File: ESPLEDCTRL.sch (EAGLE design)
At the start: 15 parts, among them IC1 74HC1G08GW

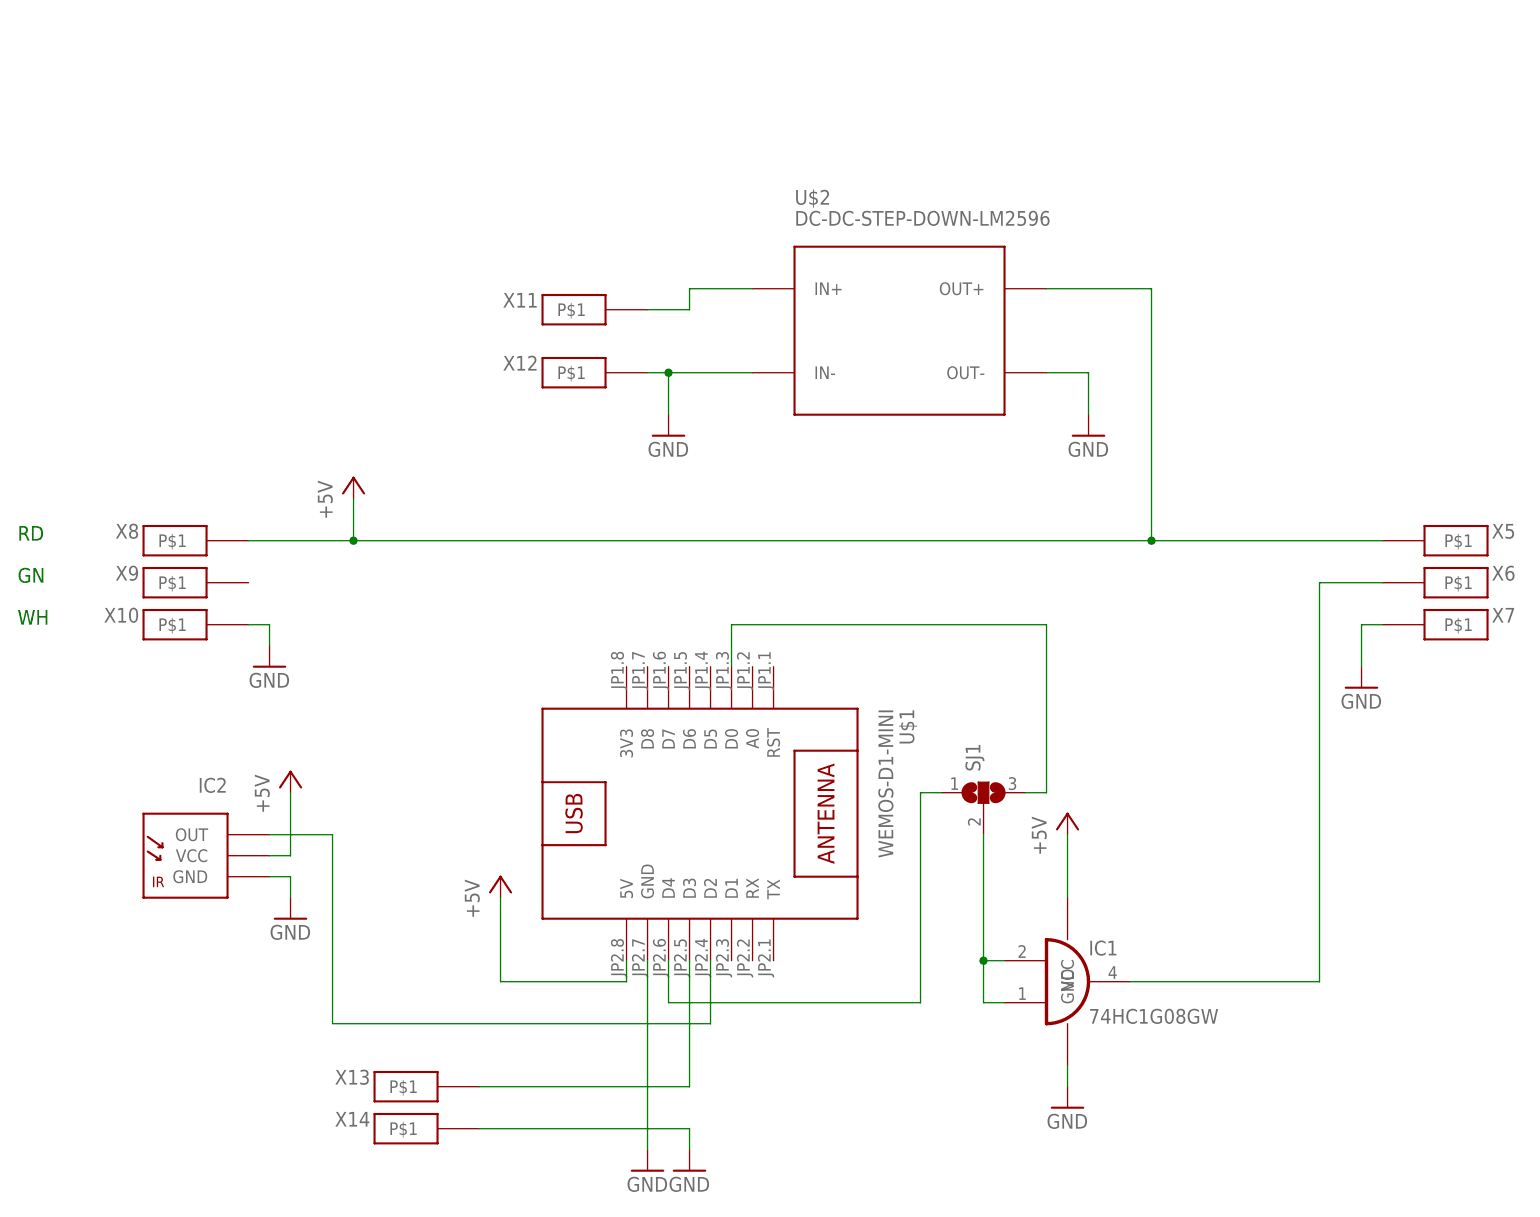
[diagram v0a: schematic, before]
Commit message: Board fertig gestellt
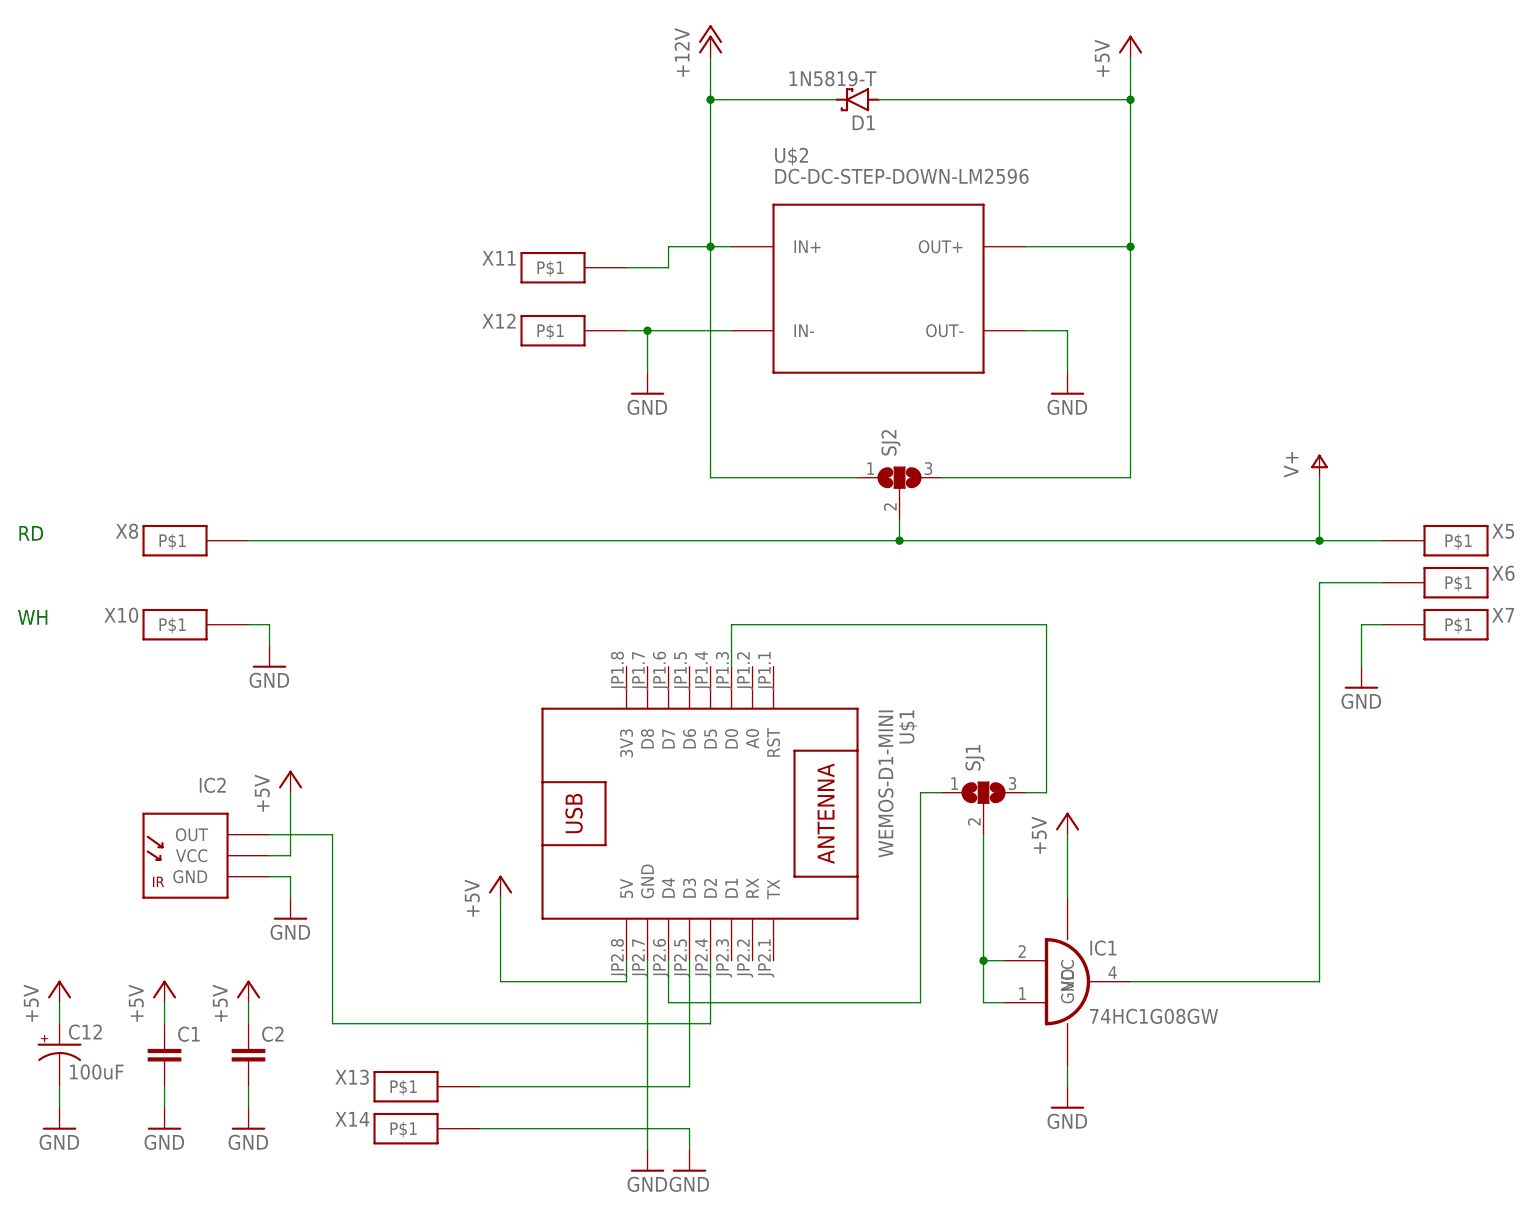
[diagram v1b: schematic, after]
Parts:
- removed X9: (no value), modules:PAD2X4
- added C1, C2: (no value), rcl:C-EUC1206
- added C12: 100uF, rcl:CPOL-USD
- added D1: 1N5819-T, diode:1N5819-T
- added SJ2: (no value), jumper:SJ2W
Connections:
- removed net N$21: U$2.IN+, X11.P$1
- new net +12V: D1.C, SJ2.1, U$2.IN+, X11.P$1
- new net V+: SJ2.2, X5.P$1, X8.P$1
- net +5V: now also C1.1, C12.+, C2.1, D1.A, SJ2.3; no longer X5.P$1, X8.P$1
- net GND: now also C1.2, C12.-, C2.2
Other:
- note removed: "GN"
- moved on the sheet: U$2, X11, X12
